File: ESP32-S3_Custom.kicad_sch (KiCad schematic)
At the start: 22 parts, among them J1 Conn_01x20_Pin, J2 Conn_01x20_Pin, J3 USB_C_Receptacle_USB2.0_16P, J4 USB_C_Receptacle_USB2.0_16P, SW1 SW_Push, SW2 SW_Push, U1 ESP32-S3-WROOM-1, U2 AMS1117-3.3, U3 CH340K

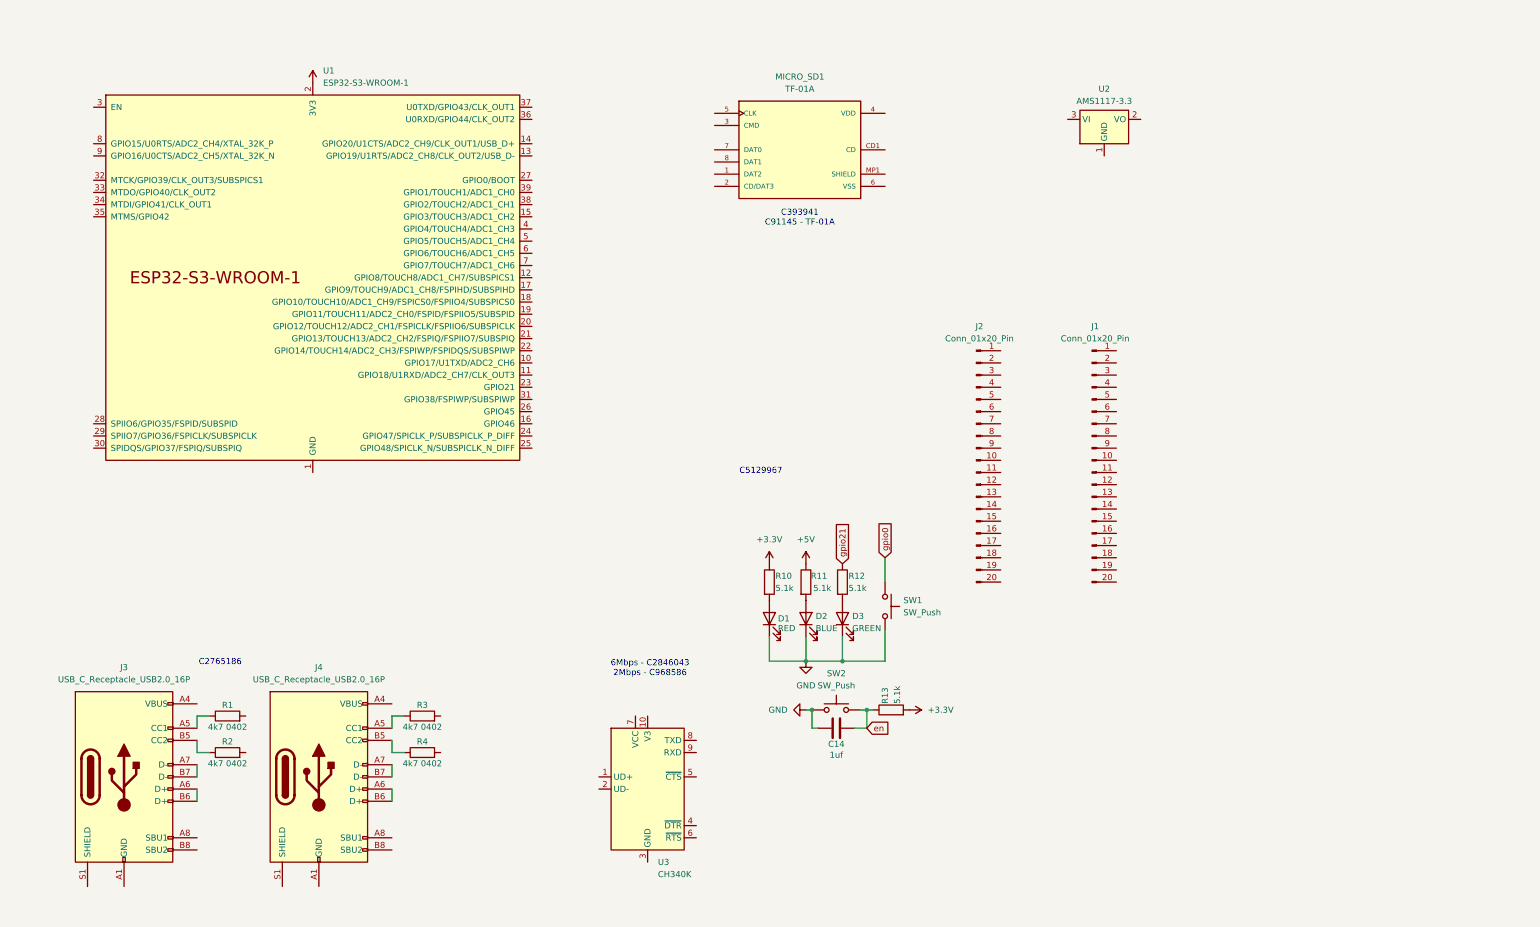
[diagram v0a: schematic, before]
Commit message: semidone
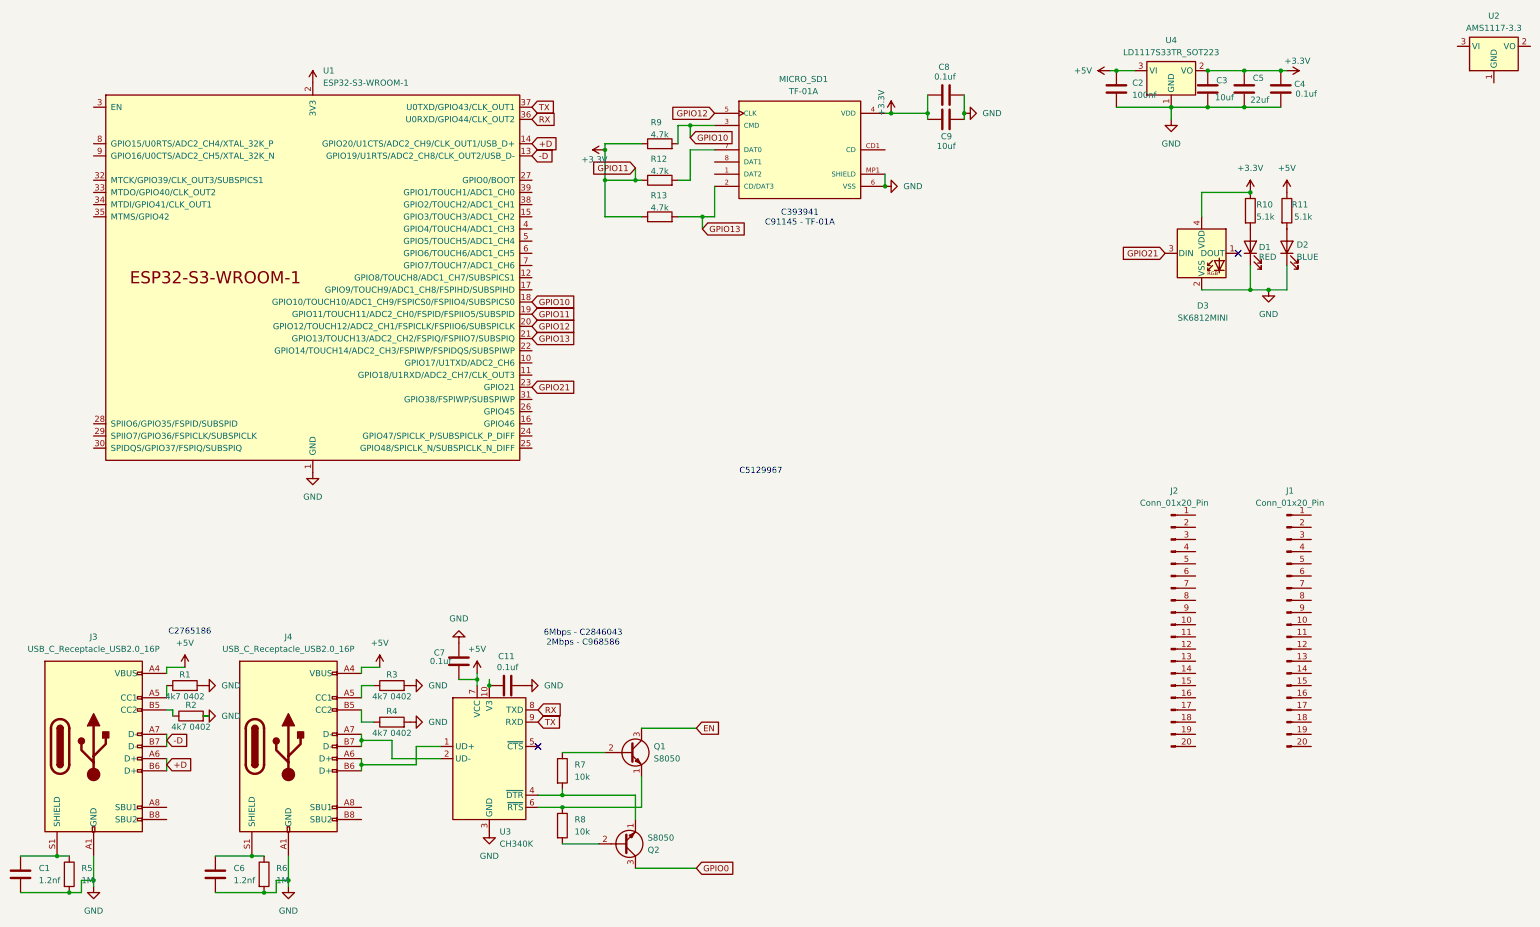
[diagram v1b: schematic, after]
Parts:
- removed C14: 1uf, symbol Device:C
- removed D3: GREEN, symbol Device:LED
- removed SW1, SW2: SW_Push, symbol Switch:SW_Push
- added C1, C6: 1.2nf, symbol Device:C
- added C11, C4, C7, C8: 0.1uf, symbol Device:C
- added C2: 100nf, symbol Device:C
- added C3, C9: 10uf, symbol Device:C
- added C5: 22uf, symbol Device:C
- added D3: SK6812MINI, LED_SMD:LED_SK6812MINI_PLCC4_3.5x3.5mm_P1.75mm, symbol LED:SK6812MINI
- added Q1, Q2: S8050, Package_TO_SOT_THT:TO-92_Inline, symbol Transistor_BJT:S8050
- added R5, R6: 1M, symbol Device:R
- added R7, R8: 10k, symbol Device:R
- added R9: 4.7k, symbol Device:R
- added U4: LD1117S33TR_SOT223, Package_TO_SOT_SMD:SOT-223-3_TabPin2, symbol Regulator_Linear:LD1117S33TR_SOT223
- R12, R13: value 5.1k -> 4.7k
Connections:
- net SHIELD is gone; now on net GND: MICRO_SD1.MP1 (SHIELD), MICRO_SD1.MP2 (SHIELD), MICRO_SD1.MP3 (SHIELD), MICRO_SD1.MP4 (SHIELD)
- net en is gone; now on net +3.3V: R13.1
- net gpio21 is gone; now on net +3.3V: R12.1
- net +3.3V: now also MICRO_SD1.4 (VDD), U1.19 (GPIO11/TOUCH11/ADC2_CH0/FSPID/FSPIIO5/SUBSPID), C3.1, C4.1, C5.1, C8.1, C9.1, D3.4 (VDD), R9.1, U4.2 (VO); no longer R13.2
- net +5V: now also J3.A4 (VBUS), J3.A9 (VBUS), J3.B4 (VBUS), J3.B9 (VBUS), J4.A4 (VBUS), J4.A9 (VBUS), J4.B4 (VBUS), J4.B9 (VBUS), U3.7 (VCC), C2.1, C7.2, U4.3 (VI)
- net GND: now also J3.A1 (GND), J3.A12 (GND), J3.B1 (GND), J3.B12 (GND), J4.A1 (GND), J4.A12 (GND), J4.B1 (GND), J4.B12 (GND), MICRO_SD1.6 (VSS), R1.2, R2.2, R3.2, R4.2, U1.1 (GND), U1.40 (GND), U1.41 (GND), U3.11 (GND), U3.3 (GND), C1.2, C11.1, C2.2, C3.2, C4.2, C5.2, C6.2, C7.1, C8.2, C9.2, D3.2 (VSS), R5.2, R6.2, U4.1 (GND)
- net at R12.2: now also MICRO_SD1.7 (DAT0)
- net -D: now reaches U1.13 (GPIO19/U1RTS/ADC2_CH8/CLK_OUT2/USB_D-)
- net -D: now also J3.A7 (D-), J3.B7 (D-)
- net +D: now reaches U1.14 (GPIO20/U1CTS/ADC2_CH9/CLK_OUT1/USB_D+)
- net +D: now also J3.A6 (D+), J3.B6 (D+)
- net GPIO10: now reaches U1.18 (GPIO10/TOUCH10/ADC1_CH9/FSPICS0/FSPIIO4/SUBSPICS0)
- net GPIO10: now also MICRO_SD1.3 (CMD), R9.2
- net GPIO12: now reaches U1.20 (GPIO12/TOUCH12/ADC2_CH1/FSPICLK/FSPIIO6/SUBSPICLK)
- net GPIO12: now also MICRO_SD1.5 (CLK)
- net GPIO13: now reaches U1.21 (GPIO13/TOUCH13/ADC2_CH2/FSPIQ/FSPIIO7/SUBSPIQ)
- net GPIO13: now also MICRO_SD1.2 (CD/DAT3), R13.2
- net GPIO21: now reaches U1.23 (GPIO21)
- net GPIO21: now also D3.3 (DIN)
- net RX: now reaches U1.36 (U0RXD/GPIO44/CLK_OUT2)
- net RX: now also U3.8 (TXD)
- net TX: now reaches U1.37 (U0TXD/GPIO43/CLK_OUT1)
- net TX: now also U3.9 (RXD)
- net at U3.1 (UD+): now also J4.A6 (D+), J4.B6 (D+)
- net at U3.10 (V3): now also C11.2
- net at U3.2 (UD-): now also J4.A7 (D-), J4.B7 (D-)
- net at U3.4 (~{DTR}): now also Q2.1 (E), R7.2
- net at U3.6 (~{RTS}): now also Q1.1 (E), R8.1
- net at J3.S1 (SHIELD): now also C1.1, R5.1
- net at J4.S1 (SHIELD): now also C6.1, R6.1
- new net: Q1.2 (B), R7.1
- new net: Q2.2 (B), R8.2
- new net EN: Q1.3 (C)
- new net GPIO0: Q2.3 (C)
- no-connect marks 0 -> 2
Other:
- moved on the sheet: D1, D2, J1, J2, J3, J4, R1, R10, R11, R2, R3, R4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
